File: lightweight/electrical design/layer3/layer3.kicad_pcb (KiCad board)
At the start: 2 copper layers, 189.7 x 105 mm, 60 parts, among them J1 SH1.0 5P, J10 SH1.0 2P, J11 SH1.0 5P, J2 SH1.0 5P, J3 SH1.0 5P, J5 Conn_01x16_Socket, J6 SH1.0 Female, SW1 SW_SPDT, SW5 SW_Push, U1 TEENSY 4.0, U2 MOUDLE-SEEEDUINO-XIAO-ESP32C3, U4 BNO085, U5 74LVC2G04, U6 74LVC2G04, U7 STM32F103C8T6, Y1 Crystal

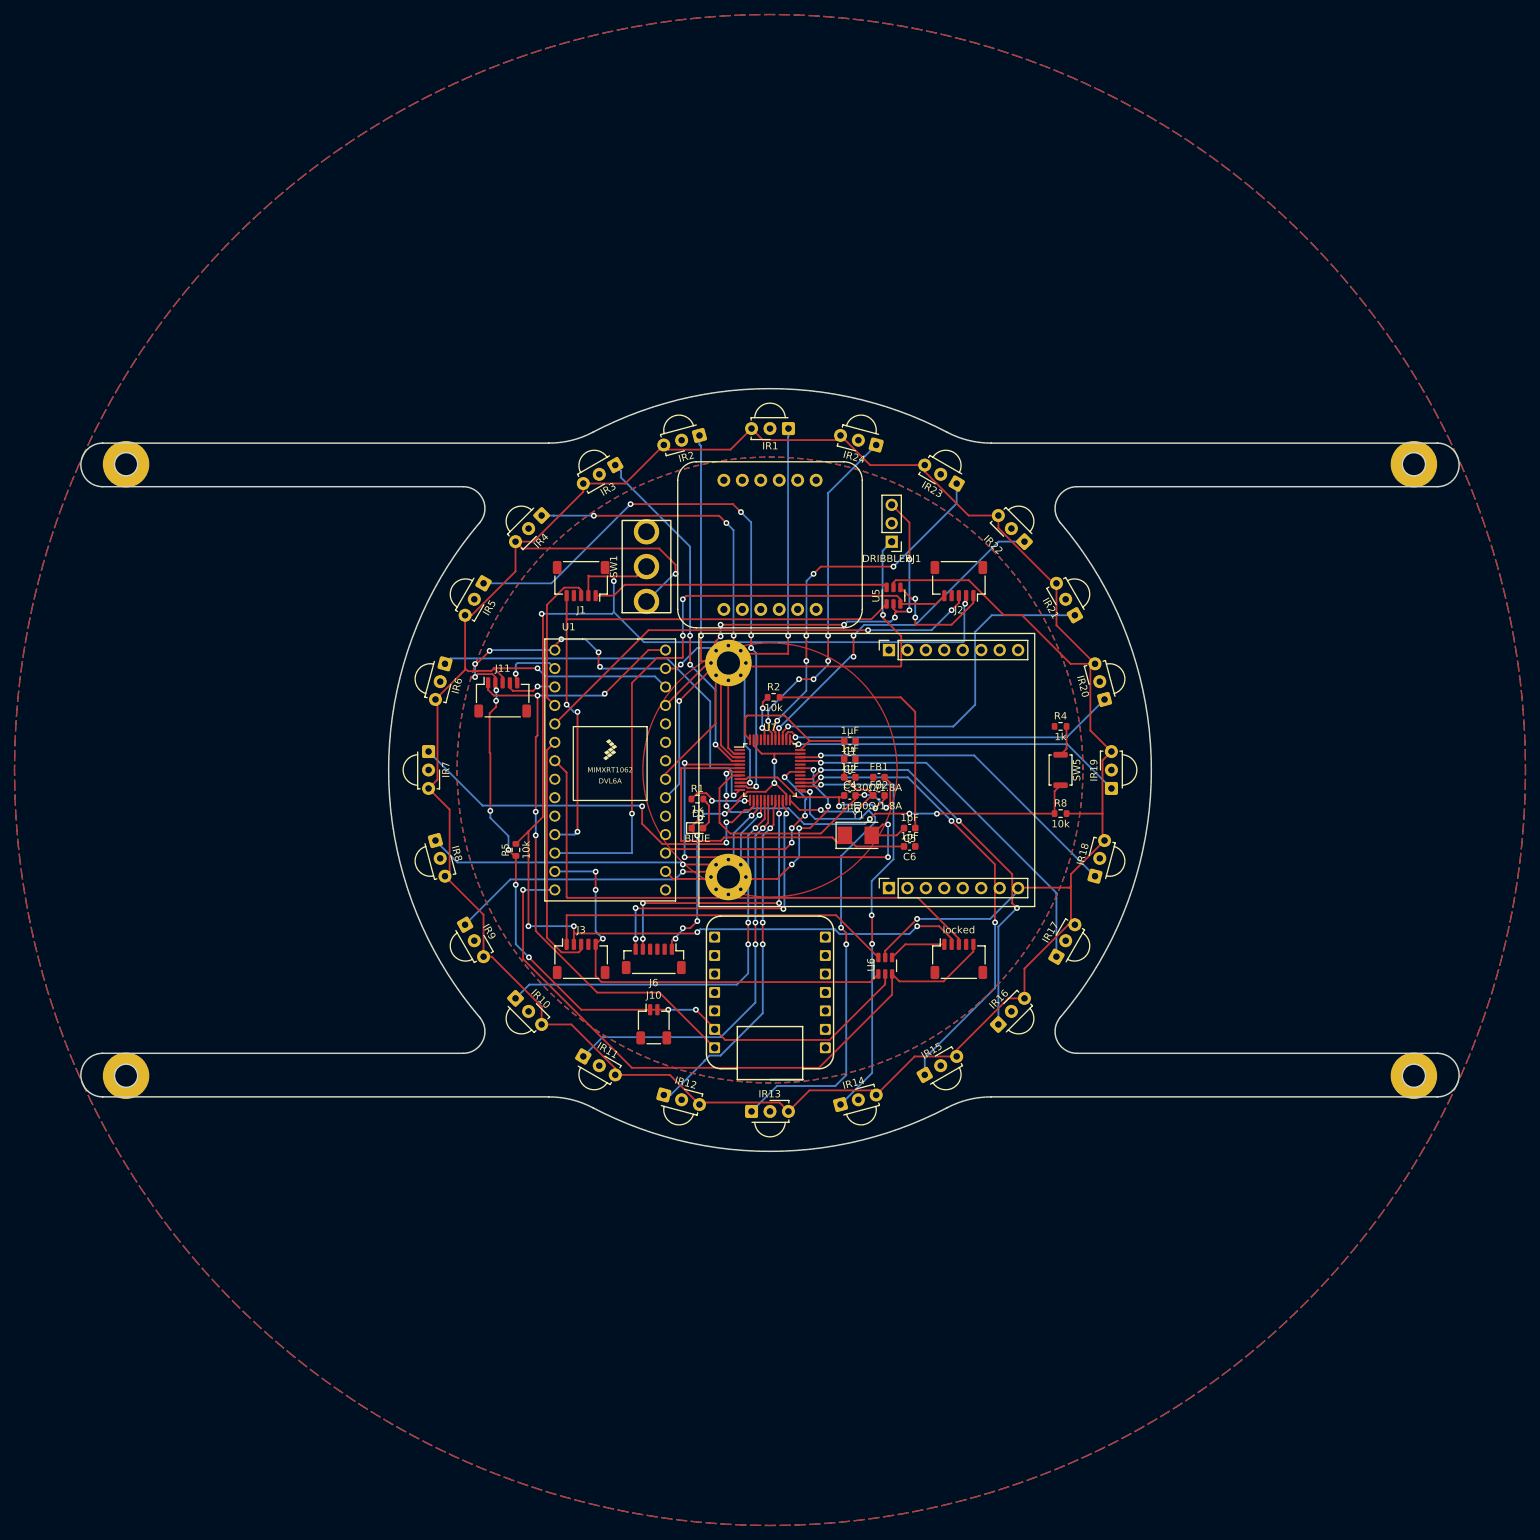
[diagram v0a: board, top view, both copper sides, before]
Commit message: update lw pcbs
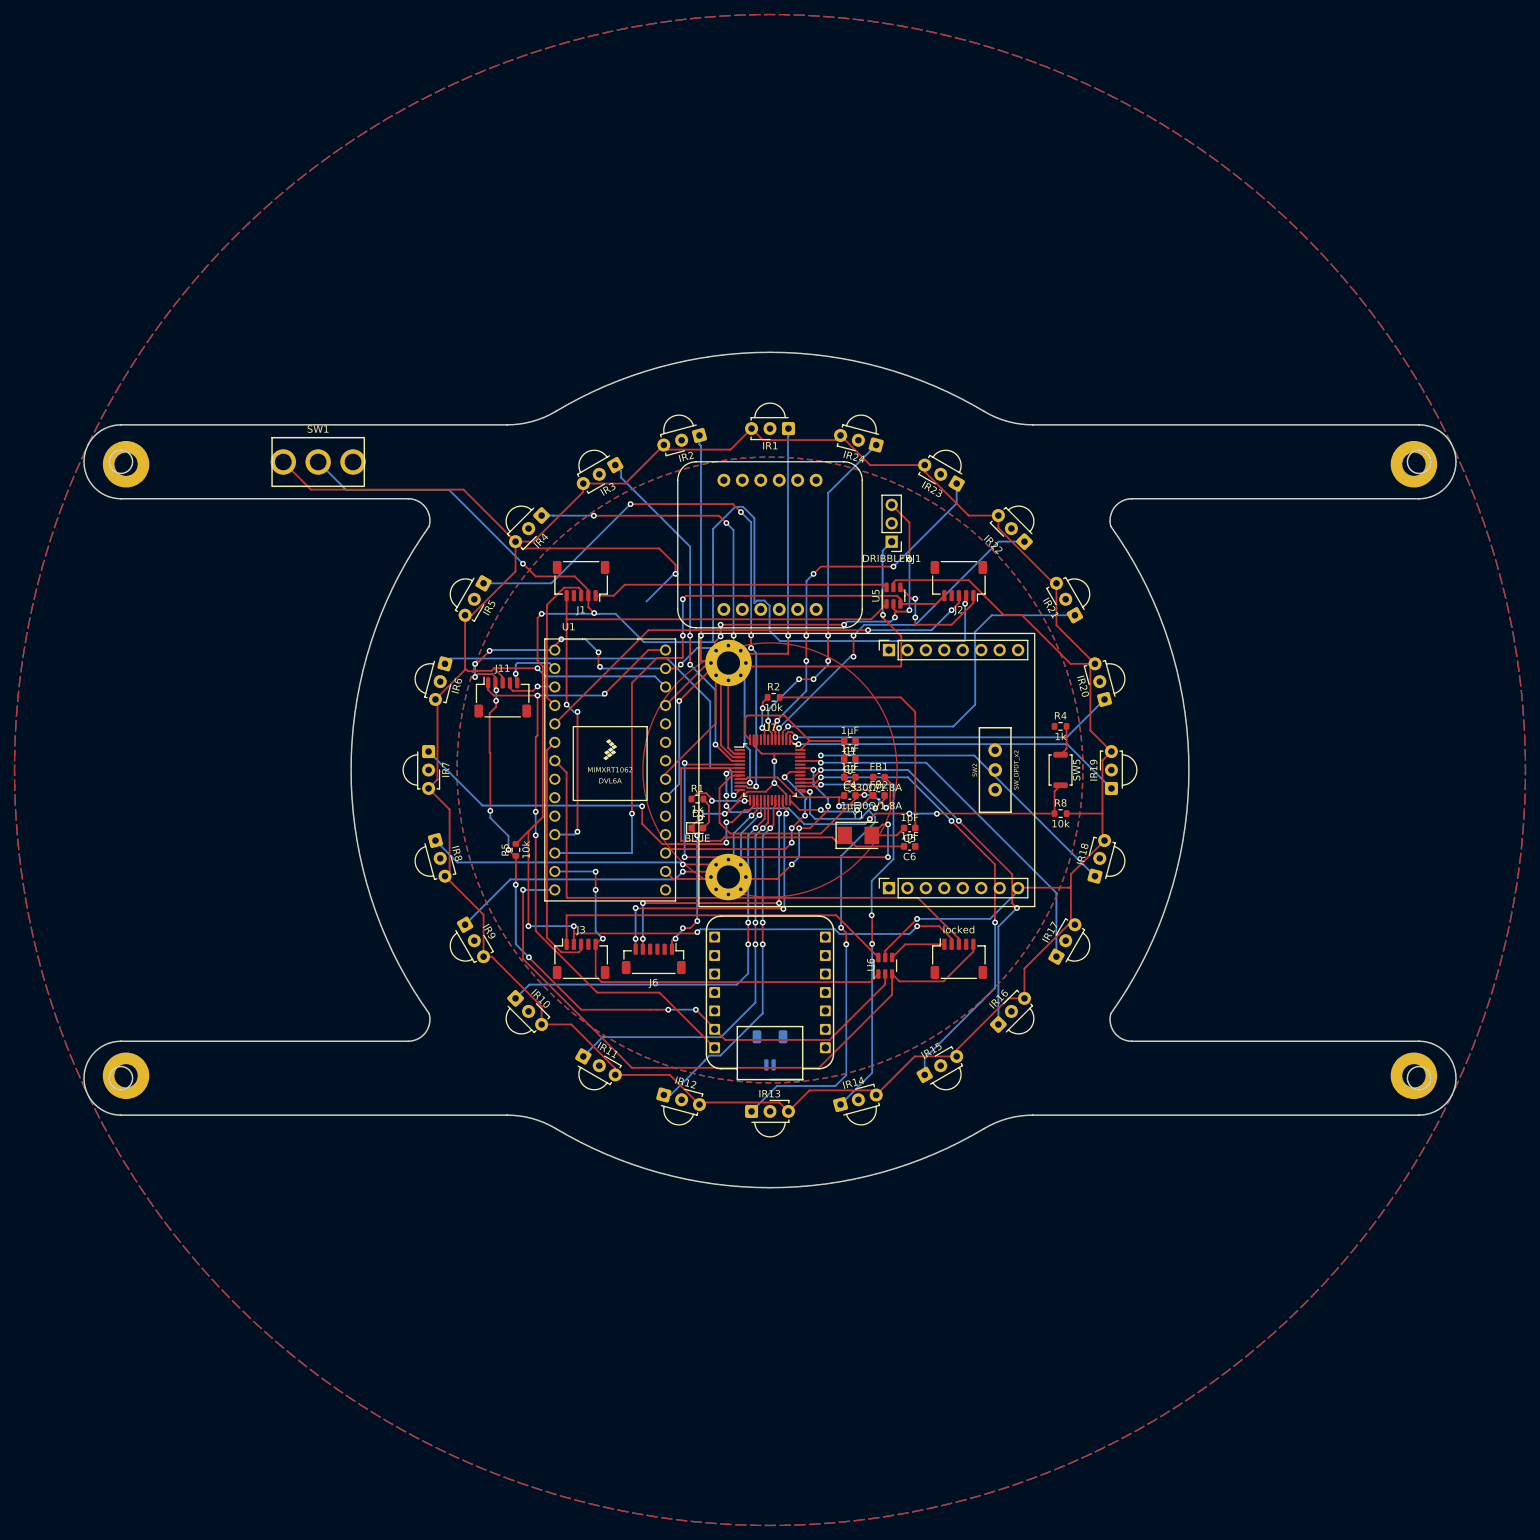
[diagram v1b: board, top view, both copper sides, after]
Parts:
- added SW2: SW_DPDT_x2, Switches:SWITCH_SPDT_PTH_11.6X4.0MM_LOCK, F.Cu at (136.0, 105.0)
- J10: moved to B.Cu
- moved SW1 47.4 mm to (42.8, 62.6), turned to 0 degrees
- moved J10 16.4 mm to (105.0, 143.6)
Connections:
- C1 pad 2: +3V3 -> /ir/MCU3V3
- C2 pad 2: +3V3 -> /ir/MCU3V3
- C3 pad 2: +3V3 -> /ir/MCU3V3
- FB2 pad 1: +3V3 -> /ir/MCU3V3
- R8 pad 2: +3V3 -> /ir/MCU3V3
- U7 pad 24: +3V3 -> /ir/MCU3V3
- U7 pad 34: /ir/IR18 -> /ir/SWDIO
- U7 pad 36: +3V3 -> /ir/MCU3V3
- U7 pad 37: /ir/IR19 -> /ir/SWDCLOCK
- U7 pad 43: unconnected-(U7-PB7-Pad43) -> /ir/IR19
- U7 pad 45: unconnected-(U7-PB8-Pad45) -> /ir/IR18
- U7 pad 48: +3V3 -> /ir/MCU3V3
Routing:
- net /EN: track 192.2 -> 258.5 mm, vias 7 -> 8
- net /ir/MCU3V3: track 0.00 -> 43.5 mm, vias 0 -> 2
- net +3V3: track 493.2 -> 486.3 mm, vias 5 -> 3
- net /ir/IR18: track 47.6 -> 45.0 mm
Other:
- board size 189.7 x 105 mm -> 188.9 x 115 mm
